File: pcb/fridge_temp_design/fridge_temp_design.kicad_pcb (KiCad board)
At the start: 2 copper layers, 66 x 63.5 mm, 12 parts, among them J1 ESP32_LEG, J2 ESP32_LEG, J3 DS18B12, J4 DS18B12, J5 DS18B12, J6 Barrel_Jack_Switch, J7 OLED

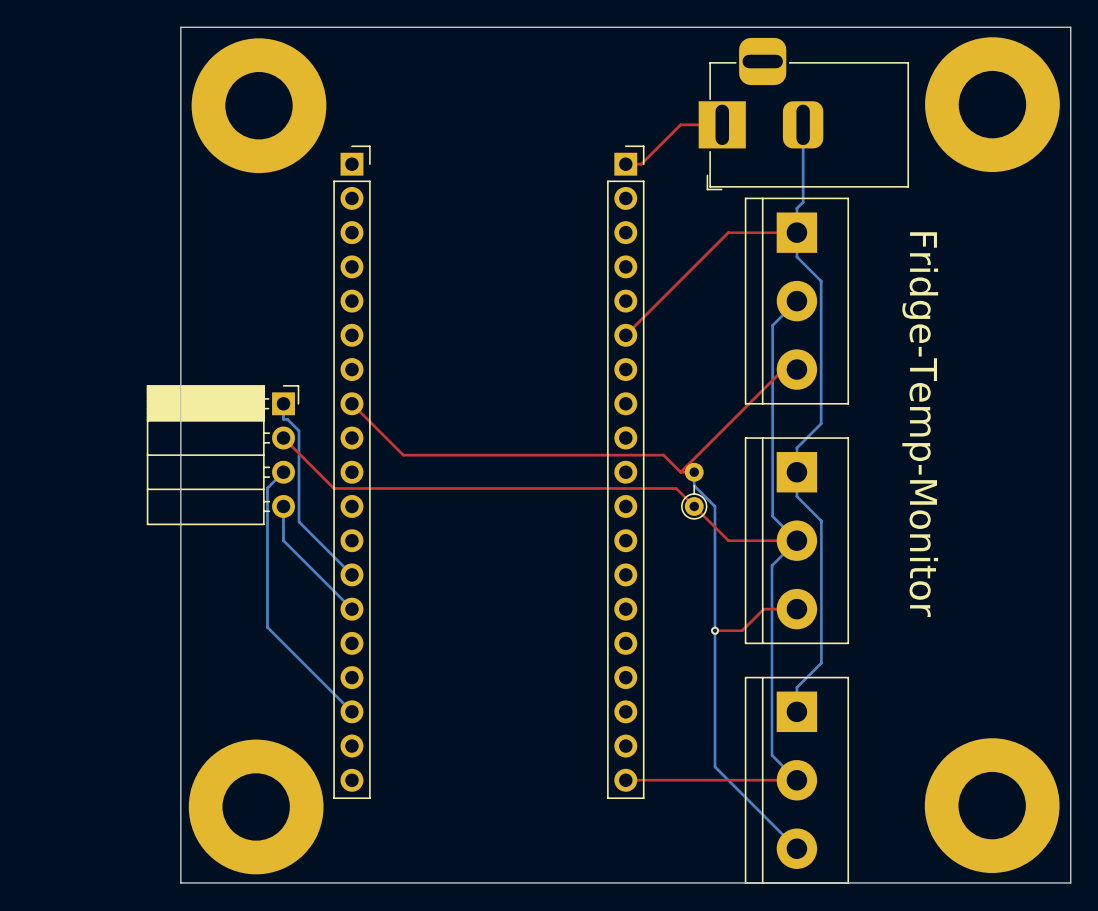
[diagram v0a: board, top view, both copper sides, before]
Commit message: v2
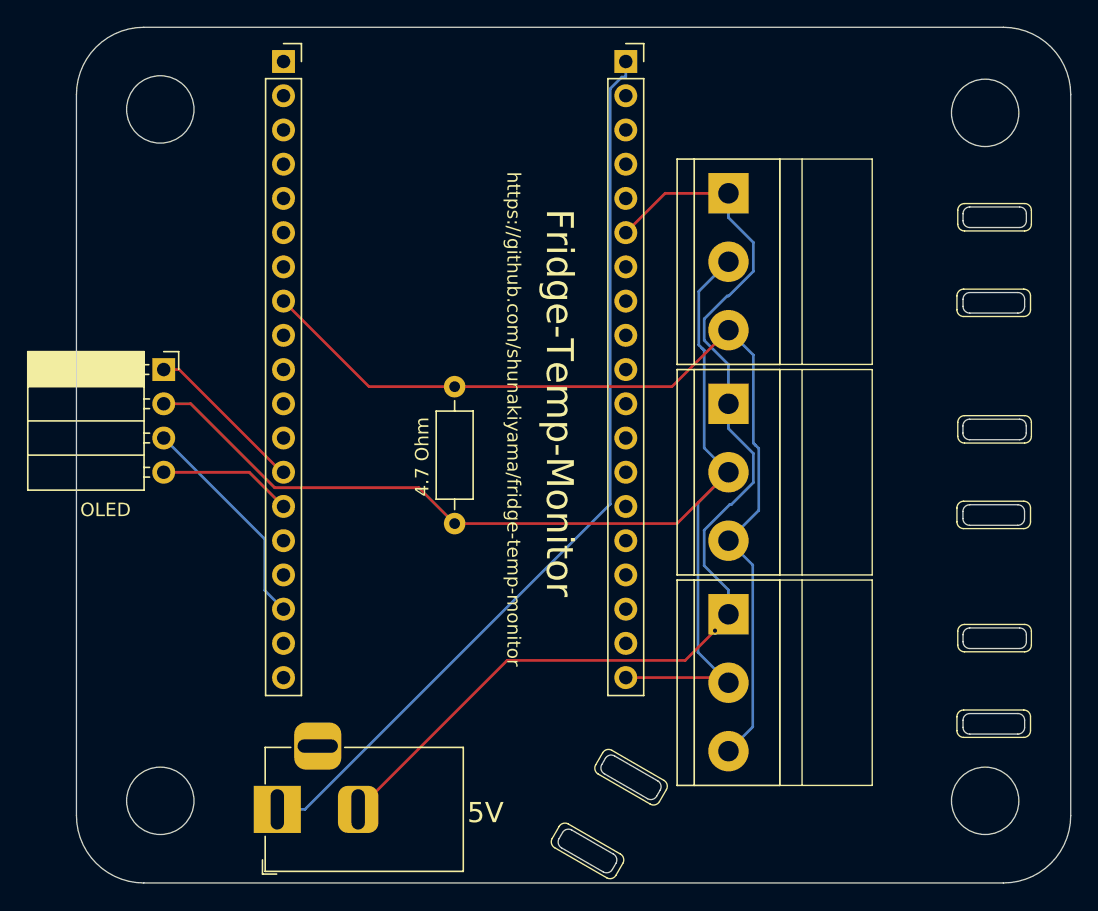
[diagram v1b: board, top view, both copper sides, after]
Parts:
- Bottom_Left, Bottom_Right, Top_Left, Top_Right: value MountingHole_5mm_Pad -> MountingHole_5mm; footprint MountingHole:MountingHole_5mm_Pad -> MountingHole:MountingHole_5mm
- R1: footprint Resistor_THT:R_Axial_DIN0204_L3.6mm_D1.6mm_P2.54mm_Vertical -> Resistor_THT:R_Axial_DIN0207_L6.3mm_D2.5mm_P10.16mm_Horizontal
- moved J6 60.6 mm to (129.1, 113.9)
- moved R1 17.8 mm to (142.2, 92.7)
- moved J7 9.25 mm to (120.7, 81.3)
- moved J2 9.16 mm to (129.5, 58.4)
- moved J5 8.84 mm to (162.6, 99.4)
- moved J1 7.62 mm to (154.9, 58.4)
- moved Top_Left 7.33 mm to (120.4, 62.0)
- moved J4 7.18 mm to (162.6, 83.8)
- moved Bottom_Left 7.13 mm to (120.4, 113.3)
- moved J3 5.86 mm to (162.6, 68.2)
- moved Top_Right 0.81 mm to (181.6, 62.2), turned to 90 degrees
- moved Bottom_Right 0.63 mm to (181.6, 113.3)
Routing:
- net Net-(J1-Pin_1): track 8.37 -> 67.6 mm
- net Net-(J1-Pin_6): track 62.6 -> 79.9 mm, vias 0 -> 1
- net Net-(J2-Pin_8): track 77.1 -> 72.2 mm, vias 1 -> 0
- net Net-(J2-Pin_17): track 20.9 -> 16.4 mm
- net Net-(J2-Pin_13): track 15.0 -> 12.0 mm
- net Net-(J1-Pin_19): track 92.5 -> 90.1 mm
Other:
- board size 66 x 63.5 mm -> 73.8 x 63.5 mm
- board text added: "4.7 Ohm"
- board text added: "5V"
- board text added: "OLED"
